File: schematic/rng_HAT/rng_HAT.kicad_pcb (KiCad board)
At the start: 2 copper layers, 25 parts, among them Q1 2N3904, Q2 2N3904, Q3 2N3904, Q4 BC107, Q5 2N3904, U1 RASPBERRY_PI_4B_4GB, U2 MAN72A, U3 STM32F103C8Tx

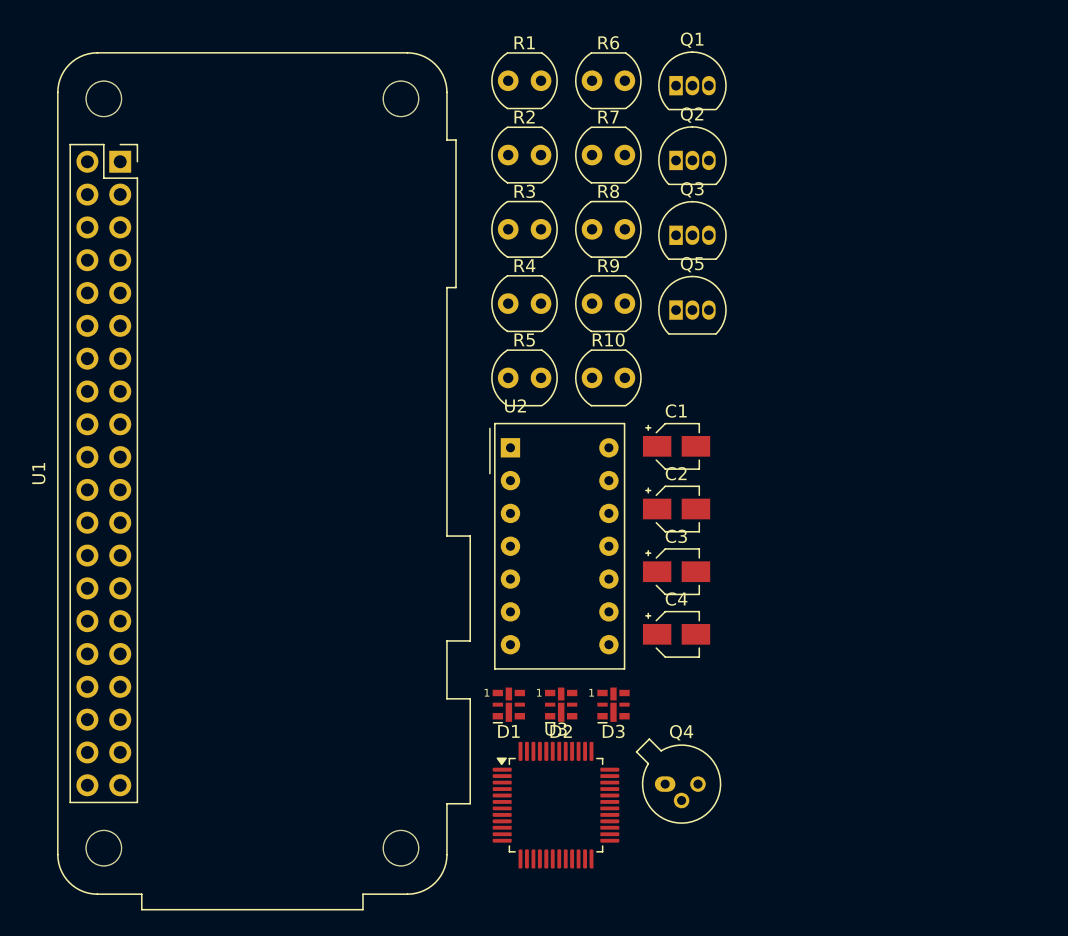
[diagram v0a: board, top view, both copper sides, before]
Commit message: working PCB?
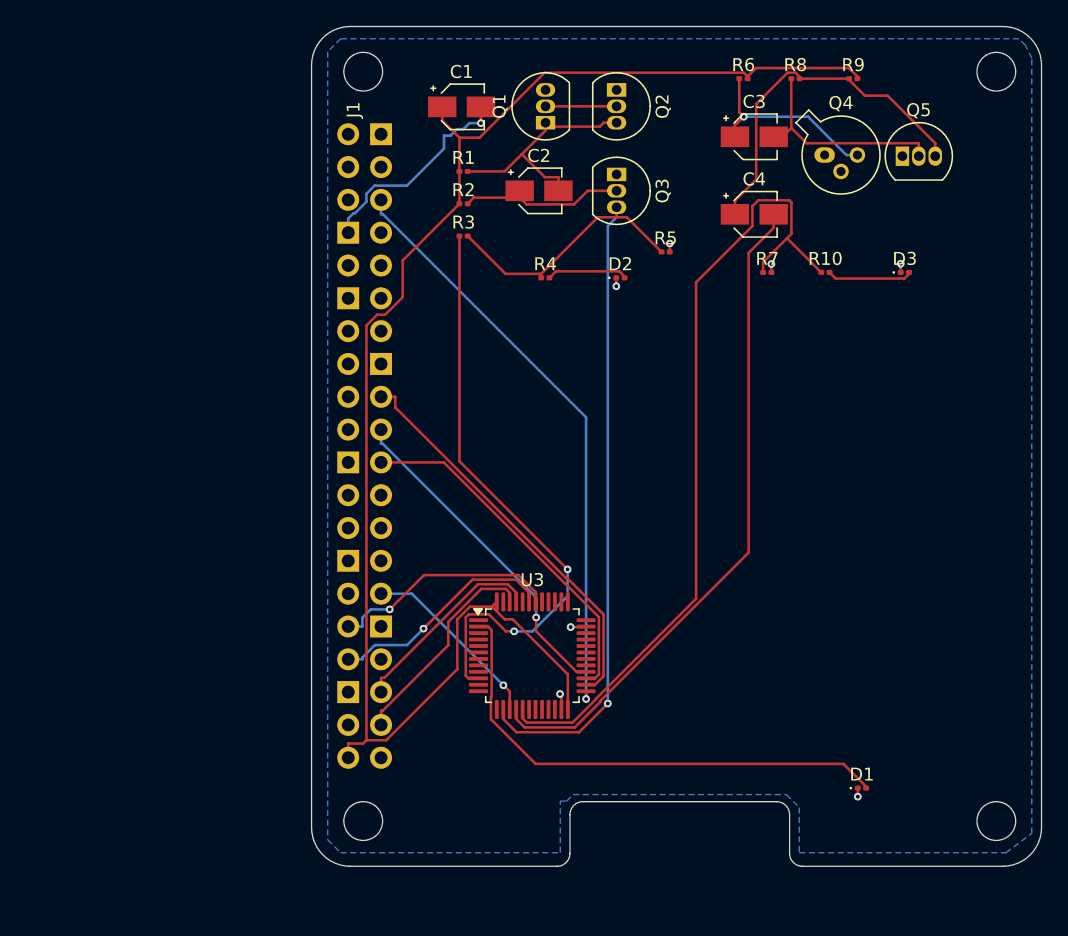
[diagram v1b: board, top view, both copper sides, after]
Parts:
- removed U1: RASPBERRY_PI_4B_4GB, Module:Raspberry_Pi_Zero_Socketed_THT_FaceDown_MountingHoles
- removed U2: MAN72A, Display_7Segment:MAN72A
- added J1: RPi_GPIO, RPI_Hat:RPI_Hat_B+, F.Cu at (143.8, 93.0)
- D1, D2, D3: footprint LED_SMD:LED-APA102-2020 -> LED_SMD:LED_0201_0603Metric
- R1, R10, R2, R3, R4, R5, R6, R7, R8, R9: footprint OptoDevice:R_LDR_4.9x4.2mm_P2.54mm_Vertical -> Resistor_SMD:R_0201_0603Metric
- moved Q4 50.2 mm to (179.5, 70.5)
- moved D3 40.3 mm to (185.7, 79.6)
- moved C3 34.2 mm to (174.0, 69.1)
- moved D2 33.4 mm to (163.7, 80.0)
- moved C4 33.1 mm to (174.0, 75.1)
- moved C1 31.1 mm to (151.4, 66.8)
- moved D1 28.1 mm to (182.3, 119.5)
- moved C2 26.8 mm to (157.4, 73.3)
- moved R9 26.7 mm to (181.7, 64.6)
- moved Q5 21.2 mm to (185.5, 70.6)
- moved R10 19.8 mm to (179.5, 79.6)
- moved R8 19.6 mm to (177.2, 64.6)
- moved R7 16.3 mm to (175.0, 79.6)
- moved R5 15.6 mm to (167.2, 78.0)
- moved R6 11.7 mm to (173.2, 64.6)
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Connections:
- U3 pad 27: STREAM B -> STRM SPI(MOSI)
- U3 pad 28: Net-(U1-GPIO9/SPI_MISO) -> STRM SPI(MISO)
- U3 pad 45: I2C_clk -> STRM I2C(CLK)
- U3 pad 46: I2C_dt -> STRM I2C(DT)
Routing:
- net 5V: track 0.00 -> 117.9 mm
- net AN LED: track 0.00 -> 69.5 mm, vias 0 -> 1
- net WN LED: track 0.00 -> 64.1 mm
- net WN OUT: track 0.00 -> 52.0 mm
- net AN OUT: track 0.00 -> 46.6 mm, vias 0 -> 2
- net CS: track 0.00 -> 45.9 mm, vias 0 -> 1
- net Net-(D1-A): track 0.00 -> 39.4 mm
- net Net-(J1-BCM11_SCLK): track 0.00 -> 31.1 mm
- net Net-(Q5-C): track 0.00 -> 27.5 mm
- net STRM SPI(MOSI): track 0.00 -> 27.4 mm
- net STRM SPI(MISO): track 0.00 -> 25.8 mm, vias 0 -> 1
- net GND: track 0.00 -> 22.9 mm, vias 0 -> 8
- net STREAM A: track 0.00 -> 18.2 mm, vias 0 -> 1
- net Net-(Q1-E): track 0.00 -> 18.2 mm
- net INTRPT?: track 0.00 -> 18.1 mm, vias 0 -> 1
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- added copper zone on B.Cu, net GND
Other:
- board outline added: 56.5 x 65 mm
